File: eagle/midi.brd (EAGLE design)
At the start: 62.5 x 83.8 mm, 33 parts, among them CON1 EXPANSION-PORT, IC1 74LS14, IC2 6N138, IC4 74LS02, IC5 74LS74, IC6 74AHCT1G32DBV, IC7 74LS273, IC8 SST39SF040, IC9 74LS00D, Q1 2MHz, Q2 DMP2100U

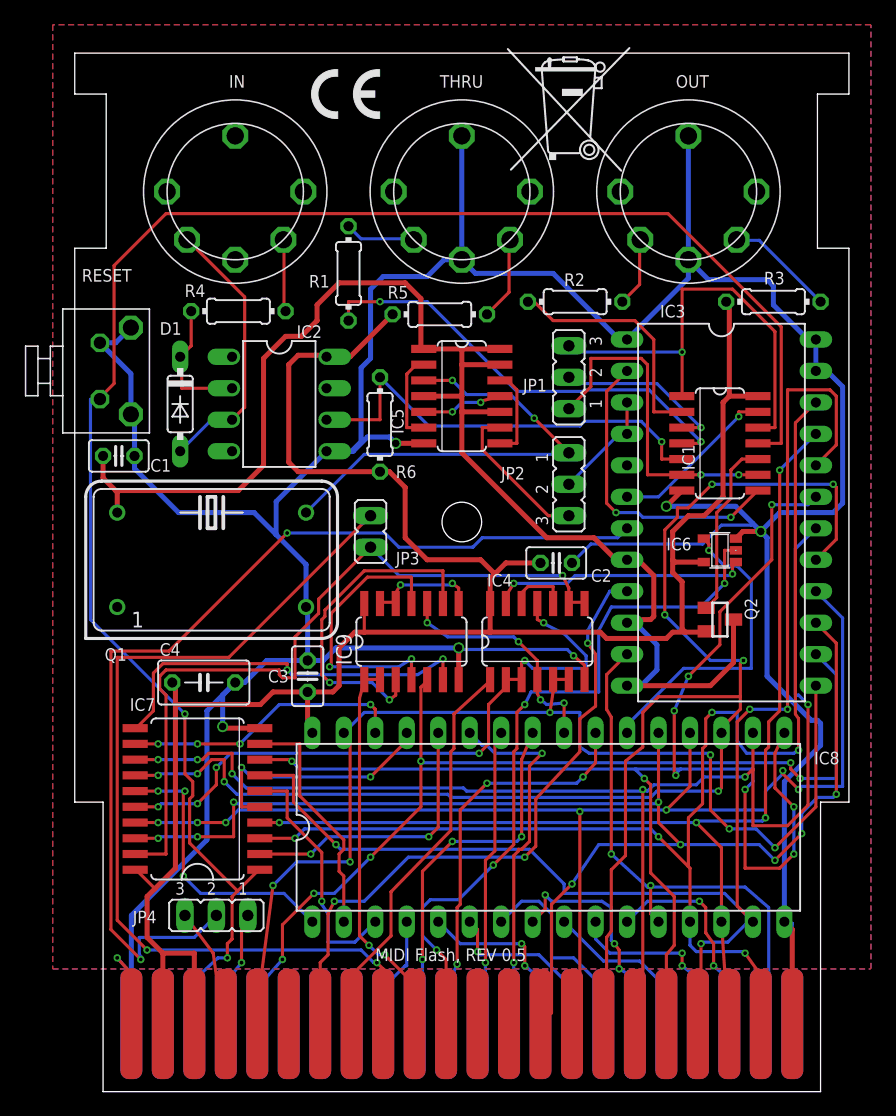
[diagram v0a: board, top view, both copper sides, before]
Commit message: revision 1.0
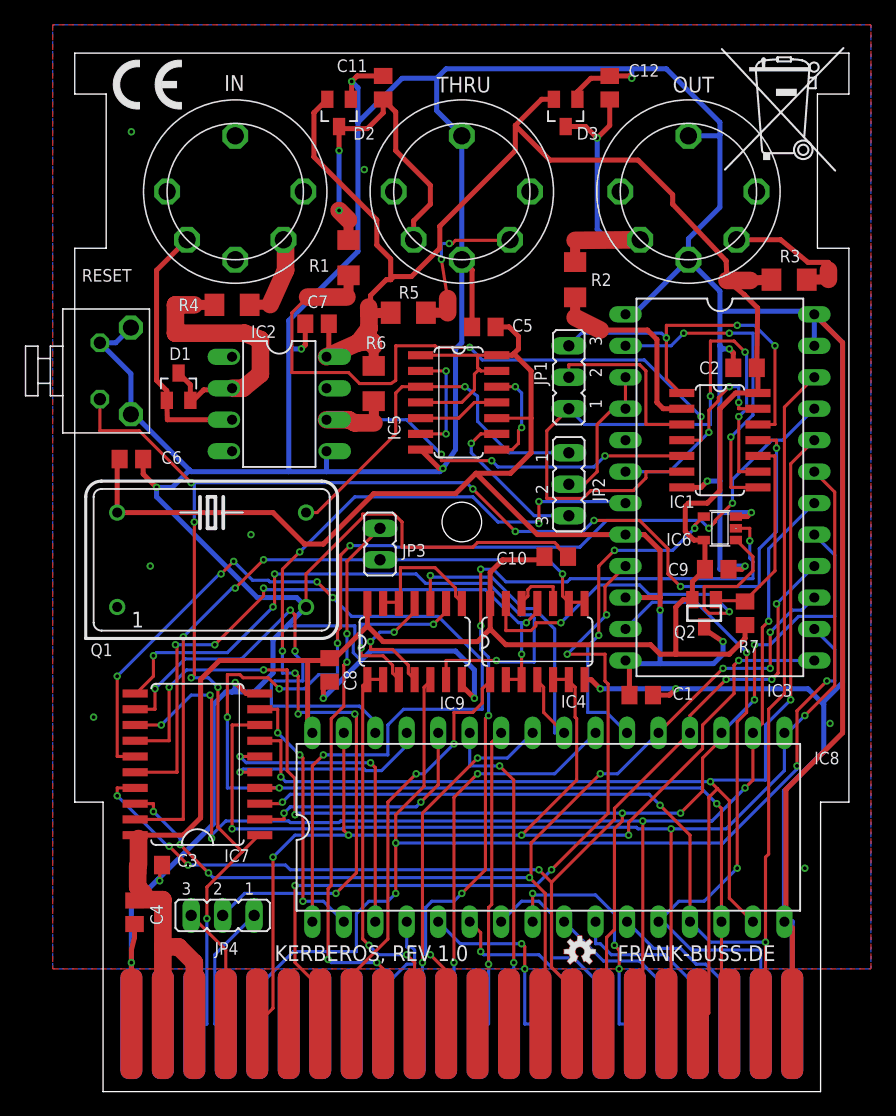
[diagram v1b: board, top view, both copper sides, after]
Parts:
- added C10, C5, C6, C7, C8, C9: 100n, rcl:C0805
- added C11, C12: 1n, rcl:C0805
- added D2, D3: BAV99, diode:SOT23
- added R7: 10k, rcl:R0805
- C1, C2, C3: device rcl:C025-025X050 -> rcl:C0805
- C4: device rcl:C050-035X075 -> rcl:C0805
- D1: value 1N914 -> BAV99; device diode:DO35-7 -> diode:SOT23
- R1, R2, R3, R4, R5, R6: device rcl:0204/7 -> rcl:R1206
- moved C1 46.4 mm to (43.7, 32.3)
- moved C2 21.9 mm to (52.1, 58.7), turned to 180 degrees
- moved C3 19.8 mm to (4.06, 18.5), turned to 0 degrees
- moved C4 19.4 mm to (2.79, 14.7), turned to 270 degrees
- moved U$1 17.3 mm to (49.5, 74.2)
- moved U$2 16.0 mm to (1.02, 79.5)
- moved R6 3.34 mm to (22.1, 57.4), turned to 90 degrees
- moved IC7 2.79 mm to (7.87, 26.7)
- moved R5 2.54 mm to (24.9, 63.1)
- moved R3 2.18 mm to (55.6, 65.8)
- moved IC3 2.04 mm to (50.0, 49.0)
- moved R2 1.78 mm to (38.4, 65.8), turned to 270 degrees
- moved IC6 1.78 mm to (50.0, 45.7)
- moved D1 1.40 mm to (6.35, 57.1), turned to 0 degrees
- moved Q2 1.37 mm to (48.8, 38.9), turned to 180 degrees
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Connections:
- removed net N$2: D1.C, IC2.2, R4.1
- new net N$37: D1.2, D1.3, IC2.2, R4.1
- net +5V: now also C10.1, C7.1, C8.1, C9.1, D2.2, D3.2, R7.1
- net 5V-SW: now also C5.1, C6.1
- net GND: now also C10.2, C11.2, C12.2, C5.2, C6.2, C7.2, C8.2, C9.2, D2.1, D3.1
- net N$16: now also C12.1, D3.3
- net N$28: now also C11.1, D2.3
- net N$3: now also D1.1; no longer D1.A
- net N$35: now also R7.2
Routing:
- net GND: track 318.6 -> 509.2 mm, vias 7 -> 23
- net N$22: track 22.9 -> 78.1 mm, vias 3 -> 6
- net +5V: track 177.3 -> 232.1 mm
- net D1: track 90.8 -> 133.5 mm, vias 4 -> 8
- net EXROM: track 73.9 -> 45.7 mm, vias 2 -> 4
- net N$5: track 27.4 -> 53.5 mm, vias 2 -> 3
- net D7: track 108.5 -> 83.2 mm, vias 9 -> 8
- net D5: track 133.6 -> 108.7 mm, vias 8 -> 7
- net N$37: track 0.00 -> 24.2 mm
- net N$28: track 5.72 -> 28.2 mm, vias 0 -> 2
- net N$23: track 31.5 -> 52.4 mm, vias 2 -> 4
- net N$16: track 5.60 -> 24.7 mm, vias 0 -> 1
- net N$12: track 36.4 -> 53.7 mm
- net RESET: track 142.7 -> 127.3 mm, vias 2 -> 10
- net D3: track 115.0 -> 99.8 mm, vias 9 -> 3
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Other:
- board text added: "FRANK-BUSS.DE"
- board text added: "KERBEROS, REV 1.0"
- board text removed: "MIDI Flash, REV 0.5"
